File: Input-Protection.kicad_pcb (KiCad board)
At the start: 2 copper layers, 59 parts, among them J101 KLDX-0202-B, J102 EBWA-02-B, J103 EBWA-02-B, J104 KLDX-0202-B, Q201 MCU18P10Y-TP, Q501 BC846, Q502 MCU18P10Y-TP, U401 LM4040DBZ-5, U601 AZV3002S-13

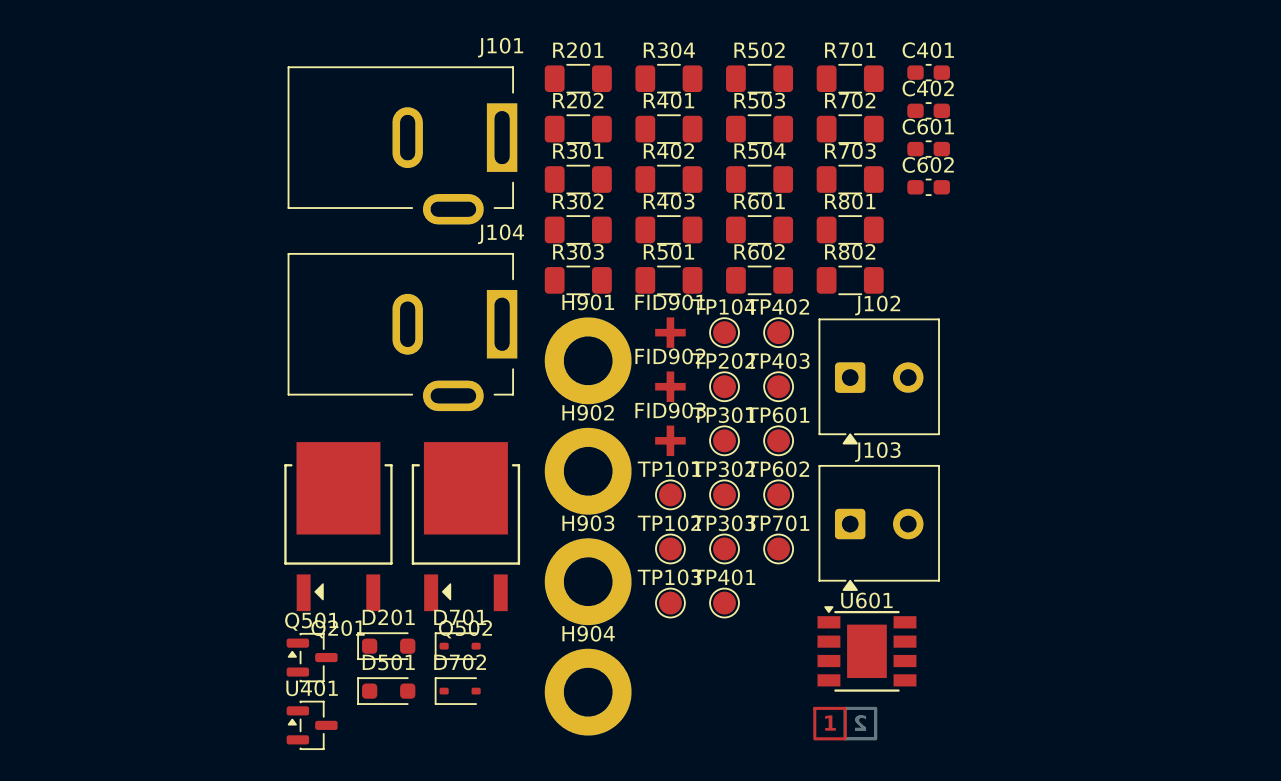
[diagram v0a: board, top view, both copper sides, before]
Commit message: feat: preliminary pcb layout
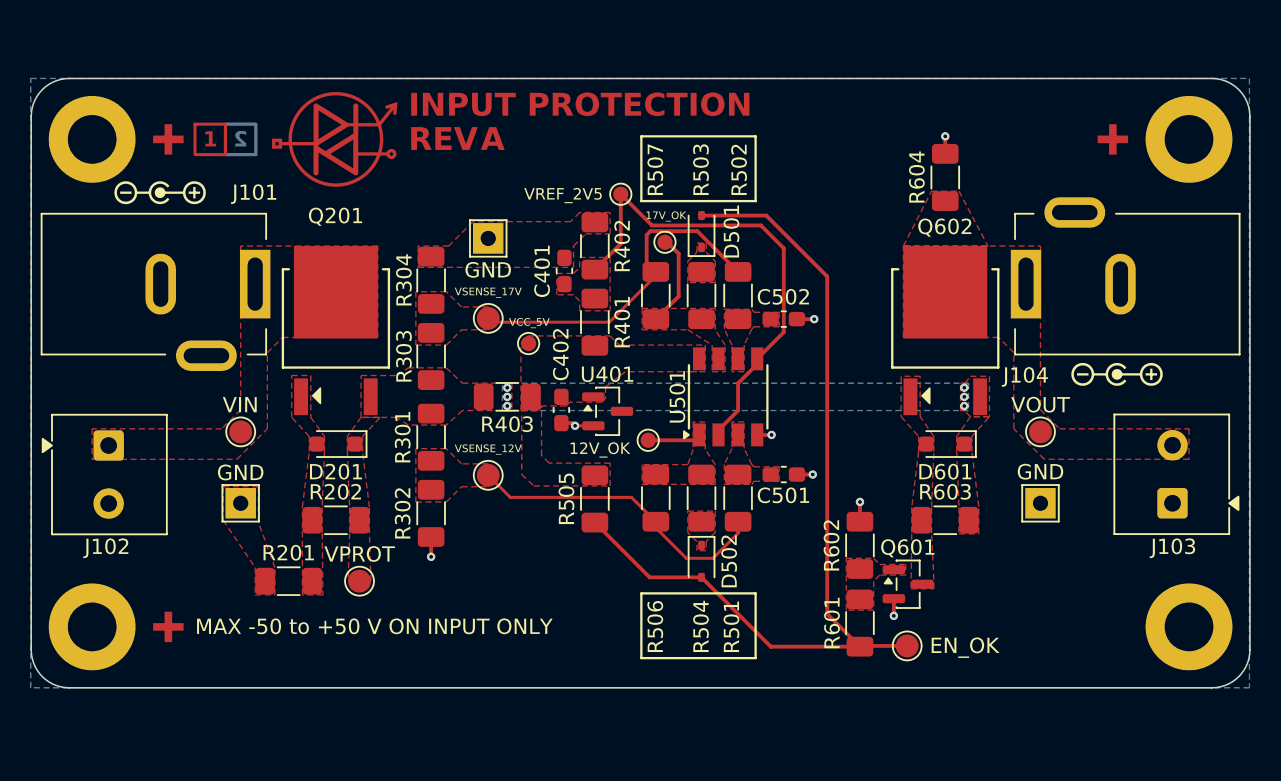
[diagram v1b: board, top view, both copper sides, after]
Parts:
- removed C601, C602: 10n, Capacitor_SMD:C_0603_1608Metric_Pad1.08x0.95mm_HandSolder
- removed D701, D702: 1N4148WS, Diode_SMD:D_SOD-323
- removed Q501: BC846, Package_TO_SOT_SMD:SOT-23
- removed Q502: MCU18P10Y-TP, MCU18P10Y-TP:DPAK_MCC
- removed R701, R702: 470, Resistor_SMD:R_1206_3216Metric_Pad1.30x1.75mm_HandSolder
- removed R703: 47k, Resistor_SMD:R_1206_3216Metric_Pad1.30x1.75mm_HandSolder
- removed R801, R802: 1M, Resistor_SMD:R_1206_3216Metric_Pad1.30x1.75mm_HandSolder
- removed TP202: VPROT, TestPoint:TestPoint_Pad_D1.5mm
- removed TP402: VCC_5V, TestPoint:TestPoint_Pad_D1.5mm
- removed TP601: 12V_OK, TestPoint:TestPoint_Pad_D1.5mm
- removed TP602: 17V_OK, TestPoint:TestPoint_Pad_D1.5mm
- removed TP701: EN_OK, TestPoint:TestPoint_Pad_D1.5mm
- removed U601: AZV3002S-13, Package_SO:Diodes_SO-8EP
- added C501: 10n, Capacitor_SMD:C_0603_1608Metric_Pad1.08x0.95mm_HandSolder, F.Cu at (161.0, 87.7)
- added C502: 10n, Capacitor_SMD:C_0603_1608Metric_Pad1.08x0.95mm_HandSolder, F.Cu at (161.0, 77.5)
- added D502: 1N4148WS, Diode_SMD:D_SOD-323, F.Cu at (155.6, 93.3)
- added D601: D3Z10BF-7, Diode_SMD:D_SOD-323_HandSoldering, F.Cu at (171.6, 85.7)
- added Q601: BC846, Package_TO_SOT_SMD:SOT-23, F.Cu at (169.1, 94.8)
- added Q602: MCU18P10Y-TP, MCU18P10Y-TP:DPAK_MCC, F.Cu at (171.6, 77.4)
- added R505: 47k, Resistor_SMD:R_1206_3216Metric_Pad1.30x1.75mm_HandSolder, F.Cu at (148.6, 89.2)
- added R506: 1M, Resistor_SMD:R_1206_3216Metric_Pad1.30x1.75mm_HandSolder, F.Cu at (152.6, 89.2)
- added R507: 1M, Resistor_SMD:R_1206_3216Metric_Pad1.30x1.75mm_HandSolder, F.Cu at (152.6, 75.9)
- added R603: 100k, Resistor_SMD:R_1206_3216Metric_Pad1.30x1.75mm_HandSolder, F.Cu at (171.6, 90.7)
- added R604: 1M, Resistor_SMD:R_1206_3216Metric_Pad1.30x1.75mm_HandSolder, F.Cu at (171.6, 68.2)
- added TP201: VPROT, TestPoint:TestPoint_Pad_D1.5mm, F.Cu at (133.1, 94.7)
- added TP501: 12V_OK, TestPoint:TestPoint_Pad_D1.0mm, F.Cu at (152.1, 85.4)
- added TP502: 17V_OK, TestPoint:TestPoint_Pad_D1.0mm, F.Cu at (153.2, 72.4)
- added TP503: EN_OK, TestPoint:TestPoint_Pad_D1.5mm, F.Cu at (169.1, 98.9)
- added U501: AZV3002S-13, Package_SO:Diodes_SO-8EP, F.Cu at (157.3, 82.5)
- D501: value D3Z10BF-7 -> 1N4148WS; footprint Diode_SMD:D_SOD-323_HandSoldering -> Diode_SMD:D_SOD-323
- R501: value 10k -> 1k
- R502: value 100k -> 1k
- R503: value 100k -> 470
- R504: value 1M -> 470
- R601: value 1k -> 10k
- R602: value 1k -> 100k
- TP101, TP104, TP301: footprint TestPoint:TestPoint_Pad_D1.5mm -> TestPoint:TestPoint_THTPad_2.0x2.0mm_Drill1.0mm
- TP401: footprint TestPoint:TestPoint_Pad_D1.5mm -> TestPoint:TestPoint_Pad_D1.0mm
- TP403: value GND -> VCC_5V; footprint TestPoint:TestPoint_Pad_D1.5mm -> TestPoint:TestPoint_Pad_D1.0mm
- U401: value LM4040DBZ-5 -> LM4040N-5.0
- moved ID901 55.9 mm to (124.3, 65.7)
- moved H903 49.0 mm to (187.6, 65.7)
- moved J102 48.9 mm to (116.6, 85.7), turned to -90 degrees
- moved H904 39.7 mm to (187.6, 97.7)
- moved R201 38.1 mm to (128.5, 94.7)
- moved FID902 36.5 mm to (120.6, 97.7)
- moved D501 36.5 mm to (155.6, 71.7), turned to 90 degrees
- moved H901 35.7 mm to (115.6, 65.7)
- moved FID901 35.3 mm to (120.6, 65.7)
- moved FID903 35.1 mm to (182.6, 65.7)
- moved J104 34.5 mm to (176.9, 75.2), turned to 180 degrees
- moved H902 34.1 mm to (115.6, 97.7)
- moved C402 31.1 mm to (146.4, 83.4), turned to -90 degrees
- moved R202 30.2 mm to (131.6, 90.7)
- moved TP102 29.2 mm to (125.3, 84.8), turned to 180 degrees
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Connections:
- net VIN renamed /ARCHITECTURE/1. INTERCONNECTS/VIN
- D201 pad 1: VPROT -> /ARCHITECTURE/2. POLARITY PROTECTION/VPROT
- D501 pad 1: VPROT -> Net-(D501-K)
- D501 pad 2: Net-(D501-A) -> /ARCHITECTURE/5. COMPARATOR/EN_OK
- J103 pad 1: VOUT -> GND
- J103 pad 2: GND -> /ARCHITECTURE/1. INTERCONNECTS/VOUT
- J104 pad 1: VOUT -> /ARCHITECTURE/1. INTERCONNECTS/VOUT
- Q201 pad 3: VPROT -> /ARCHITECTURE/2. POLARITY PROTECTION/VPROT
- R202 pad 2: VPROT -> /ARCHITECTURE/2. POLARITY PROTECTION/VPROT
- R301 pad 1: VSENSE_12V -> /ARCHITECTURE/3. SENSING/VSENSE_12V
- R301 pad 2: VPROT -> /ARCHITECTURE/2. POLARITY PROTECTION/VPROT
- R302 pad 2: VSENSE_12V -> /ARCHITECTURE/3. SENSING/VSENSE_12V
- R303 pad 1: VSENSE_17V -> /ARCHITECTURE/3. SENSING/VSENSE_17V
- R303 pad 2: VPROT -> /ARCHITECTURE/2. POLARITY PROTECTION/VPROT
- R304 pad 2: VSENSE_17V -> /ARCHITECTURE/3. SENSING/VSENSE_17V
- R403 pad 2: VPROT -> /ARCHITECTURE/2. POLARITY PROTECTION/VPROT
- R501 pad 1: Net-(Q501-B) -> Net-(U501A-+)
- R501 pad 2: EN_OK -> /ARCHITECTURE/3. SENSING/VSENSE_12V
- R502 pad 1: Net-(Q501-B) -> Net-(U501B--)
- R502 pad 2: GND -> /ARCHITECTURE/3. SENSING/VSENSE_17V
- R503 pad 1: Net-(D501-A) -> Net-(D501-K)
- R503 pad 2: VPROT -> /ARCHITECTURE/5. COMPARATOR/17V_OK
- R504 pad 1: VOUT -> Net-(D502-K)
- R504 pad 2: GND -> /ARCHITECTURE/5. COMPARATOR/12V_OK
- R601 pad 1: Net-(U601A-+) -> Net-(Q601-B)
- R601 pad 2: VSENSE_12V -> /ARCHITECTURE/5. COMPARATOR/EN_OK
- R602 pad 1: Net-(U601B--) -> Net-(Q601-B)
- R602 pad 2: VSENSE_17V -> GND
- TP103 pad 1: VOUT -> /ARCHITECTURE/1. INTERCONNECTS/VOUT
- TP302 pad 1: VSENSE_12V -> /ARCHITECTURE/3. SENSING/VSENSE_12V
- TP303 pad 1: VSENSE_17V -> /ARCHITECTURE/3. SENSING/VSENSE_17V
- TP403 pad 1: GND -> VCC_5V
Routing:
- net /ARCHITECTURE/5. COMPARATOR/EN_OK: track 0.00 -> 59.5 mm
- net VREF_2V5: track 0.00 -> 31.8 mm
- net /ARCHITECTURE/3. SENSING/VSENSE_17V: track 0.00 -> 22.6 mm
- net /ARCHITECTURE/3. SENSING/VSENSE_12V: track 0.00 -> 20.3 mm
- net GND: track 0.00 -> 10.2 mm, vias 0 -> 8
- net /ARCHITECTURE/5. COMPARATOR/17V_OK: track 0.00 -> 5.98 mm
- net /ARCHITECTURE/5. COMPARATOR/12V_OK: track 0.00 -> 3.49 mm
- net /ARCHITECTURE/2. POLARITY PROTECTION/VPROT: vias 0 -> 6
- added copper zone on F.Cu, net /ARCHITECTURE/1. INTERCONNECTS/VIN
- added copper zone on F.Cu, net /ARCHITECTURE/1. INTERCONNECTS/VOUT
- added copper zone on B.Cu, net /ARCHITECTURE/2. POLARITY PROTECTION/VPROT
- added copper zone on F.Cu, net /ARCHITECTURE/2. POLARITY PROTECTION/VPROT
- added copper zone on F.Cu, net /ARCHITECTURE/3. SENSING/VSENSE_12V
- added copper zone on F.Cu, net /ARCHITECTURE/3. SENSING/VSENSE_17V
- added copper zone on F.Cu, net /ARCHITECTURE/5. COMPARATOR/12V_OK
- added copper zone on F.Cu, net /ARCHITECTURE/5. COMPARATOR/17V_OK
- added copper zone on B.Cu, net GND
- added copper zone on F.Cu, net GND
- added copper zone on F.Cu, net Net-(D201-A)
- added copper zone on F.Cu, net Net-(D501-K)
- added copper zone on F.Cu, net Net-(D502-K)
- added copper zone on F.Cu, net Net-(D601-A)
- added copper zone on F.Cu, net Net-(Q601-B)
- added copper zone on F.Cu, net Net-(U501A-+)
- added copper zone on F.Cu, net Net-(U501B--)
- added copper zone on F.Cu, net VCC_5V
- added copper zone on F.Cu, net VREF_2V5
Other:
- board outline added: 80 x 40 mm
- board text added: "A"
- board text added: "INPUT PROTECTION"
- board text added: "MAX -50 to +50 V ON INPUT ONLY"
- board text added: "REV"

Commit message: fix: template issue
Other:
- board text removed: "Impedance Table"
